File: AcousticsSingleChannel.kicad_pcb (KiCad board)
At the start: 4 copper layers, 25.4 x 25.4 mm, 35 parts, among them J1 Conn_01x04_Pin, J2 Conn_01x04_Pin, J4 Conn_01x09_Pin, U1 OPA1604AIPWR, U2 ADS127L21IRUKT, U3 LTC6910-3CTS8#TRPBF

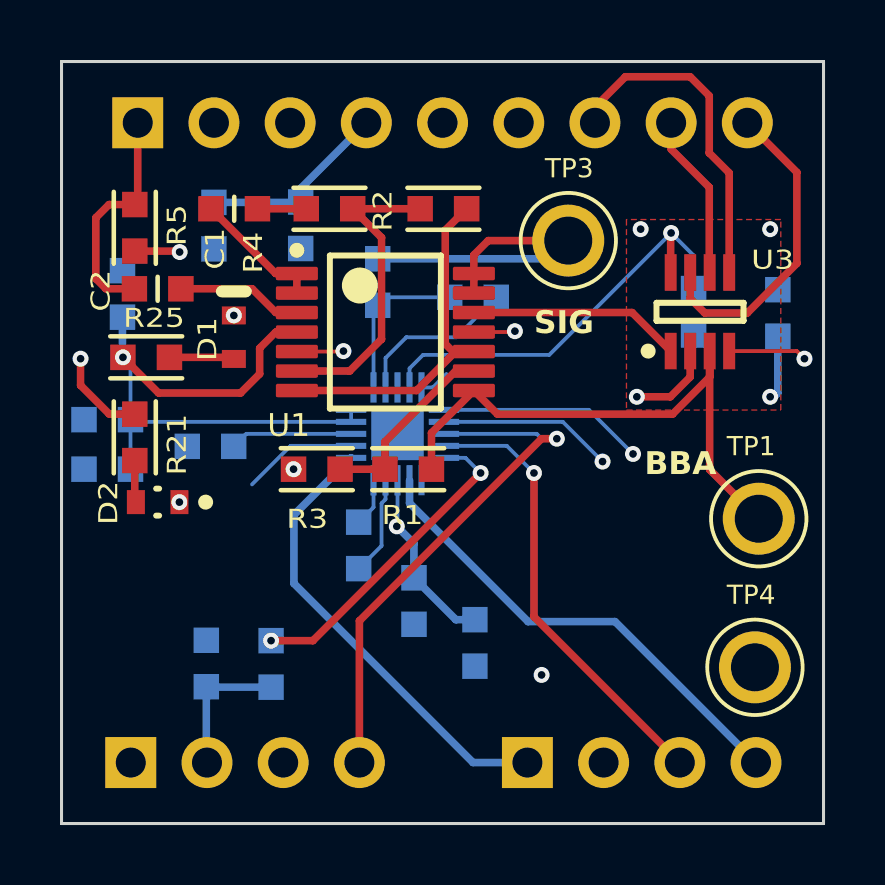
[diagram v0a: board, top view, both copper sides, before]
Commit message: tracks
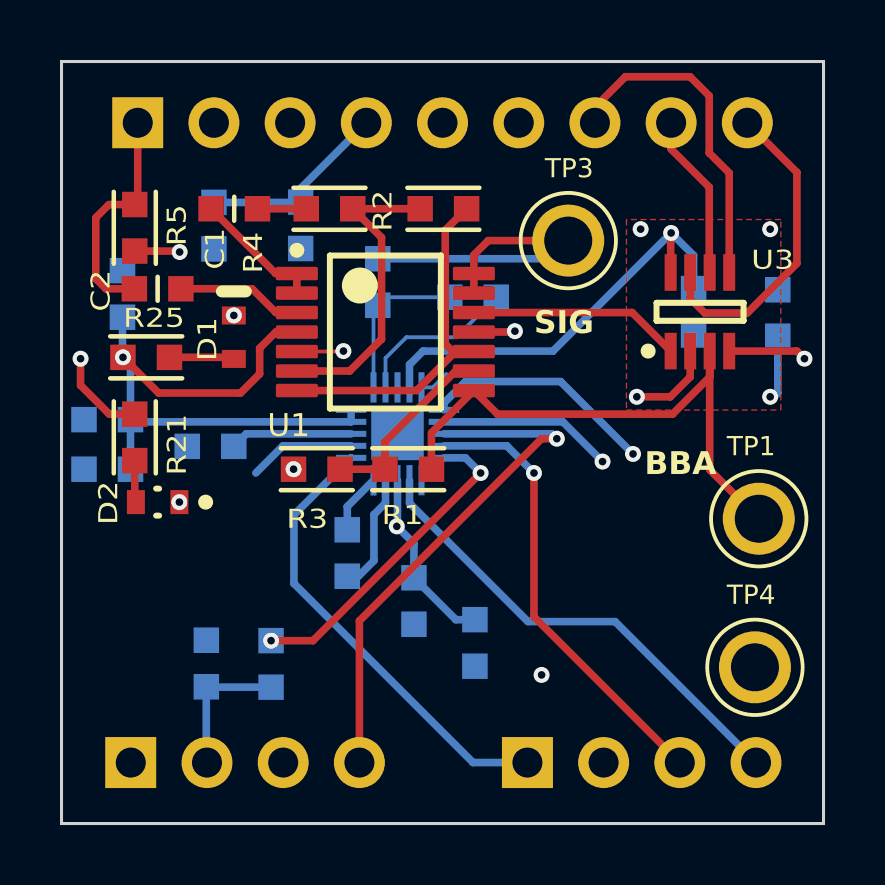
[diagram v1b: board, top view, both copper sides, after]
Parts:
- moved C4 0.46 mm to (138.3, 99.1)
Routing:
- net /RESET: track 23.8 -> 24.7 mm
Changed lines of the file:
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@@
 	(footprint "AltiumImports:SMD-0603C"
 		(layer "B.Cu")
-		(at 138.72206 98.855005 180)
+		(at 138.34106 99.109005 180)
 		(property "Reference" "C4"
 			(at 0.762 -0.635 0)
@@
 	)
 	(segment
-		(start 143.900359 91.743005)
-		(end 142.56106 91.743005)
-		(width 0.127)
+		(start 151.07106 92.378005)
+		(end 153.32706 92.378005)
+		(width 0.254)
 		(layer "F.Cu")
 		(net 1)
 	)
 	(segment
-		(start 143.92906 91.714304)
-		(end 143.900359 91.743005)
-		(width 0.127)
+		(start 143.900359 91.743005)
+		(end 143.92906 91.714304)
+		(width 0.254)
 		(layer "F.Cu")
 		(net 1)
 	)
 	(segment
-		(start 151.11798 92.424925)
-		(end 151.07106 92.378005)
+		(start 153.32706 92.378005)
+		(end 153.58106 92.632005)
 		(width 0.254)
 		(layer "F.Cu")
@@
 	)
 	(segment
-		(start 153.32706 92.378005)
+		(start 151.11798 92.424925)
 		(end 151.07106 92.378005)
-		(width 0.127)
+		(width 0.254)
 		(layer "F.Cu")
 		(net 1)
 	)
 	(segment
-		(start 153.58106 92.632005)
-		(end 153.32706 92.378005)
-		(width 0.127)
+		(start 142.56106 91.743005)
+		(end 143.900359 91.743005)
+		(width 0.254)
 		(layer "F.Cu")
 		(net 1)
@@
 	)
 	(segment
-		(start 138.72206 99.630005)
-		(end 139.48406 98.868005)
-		(width 0.127)
-		(layer "B.Cu")
-		(net 1)
-	)
-	(segment
 		(start 140.31056 91.916504)
 		(end 141.97456 91.916504)
@@
 	)
 	(segment
-		(start 139.48406 97.450006)
-		(end 139.615861 97.318205)
-		(width 0.127)
-		(layer "B.Cu")
-		(net 1)
-	)
-	(segment
 		(start 141.97456 91.916504)
 		(end 143.30706 90.584004)
@@
 	)
 	(segment
+		(start 138.70906 99.884005)
+		(end 139.23006 99.363005)
+		(width 0.254)
+		(layer "B.Cu")
+		(net 1)
+	)
+	(segment
 		(start 139.615861 93.589205)
 		(end 139.615861 92.611203)
@@
 	)
 	(segment
-		(start 136.452061 95.537004)
-		(end 135.16606 96.823005)
-		(width 0.127)
+		(start 139.23006 97.825807)
+		(end 139.615861 97.440006)
+		(width 0.254)
 		(layer "B.Cu")
 		(net 1)
 	)
 	(segment
-		(start 139.615861 97.318205)
+		(start 138.46806 95.537004)
+		(end 136.198061 95.537004)
+		(width 0.254)
+		(layer "B.Cu")
+		(net 1)
+	)
+	(segment
+		(start 139.615861 97.440006)
 		(end 139.615861 96.684805)
-		(width 0.127)
+		(width 0.254)
 		(layer "B.Cu")
 		(net 1)
 	)
 	(segment
-		(start 139.48406 98.868005)
-		(end 139.48406 97.450006)
-		(width 0.127)
+		(start 136.198061 95.537004)
+		(end 135.29306 96.442005)
+		(width 0.254)
 		(layer "B.Cu")
 		(net 1)
 	)
 	(segment
-		(start 138.46806 95.537004)
-		(end 136.452061 95.537004)
-		(width 0.127)
+		(start 138.34106 99.884005)
+		(end 138.70906 99.884005)
+		(width 0.254)
+		(layer "B.Cu")
+		(net 1)
+	)
+	(segment
+		(start 139.23006 99.363005)
+		(end 139.23006 97.825807)
+		(width 0.254)
 		(layer "B.Cu")
 		(net 1)
@@
 	)
 	(segment
-		(start 134.97306 95.137005)
-		(end 134.55706 95.553005)
-		(width 0.127)
+		(start 138.46806 95.137005)
+		(end 134.97306 95.137005)
+		(width 0.254)
 		(layer "B.Cu")
 		(net 6)
 	)
 	(segment
-		(start 138.46806 95.137005)
-		(end 134.97306 95.137005)
-		(width 0.127)
+		(start 134.97306 95.137005)
+		(end 134.55706 95.553005)
+		(width 0.254)
 		(layer "B.Cu")
 		(net 6)
 	)
 	(segment
-		(start 139.215859 96.684805)
-		(end 139.215859 97.586206)
-		(width 0.127)
+		(start 138.34106 97.559604)
+		(end 139.215859 96.684805)
+		(width 0.254)
 		(layer "B.Cu")
 		(net 7)
 	)
 	(segment
-		(start 139.215859 97.586206)
-		(end 138.72206 98.080005)
-		(width 0.127)
+		(start 138.34106 98.334005)
+		(end 138.34106 97.559604)
+		(width 0.254)
 		(layer "B.Cu")
 		(net 7)
@@
 		(start 143.659059 95.537004)
 		(end 144.56406 96.442005)
-		(width 0.127)
+		(width 0.254)
 		(layer "B.Cu")
 		(net 10)
@@
 		(start 141.56366 95.537004)
 		(end 143.659059 95.537004)
-		(width 0.127)
+		(width 0.254)
 		(layer "B.Cu")
 		(net 10)
@@
 		(start 141.56366 94.737006)
 		(end 145.526061 94.737006)
-		(width 0.127)
+		(width 0.254)
 		(layer "B.Cu")
 		(net 11)
@@
 		(start 145.526061 94.737006)
 		(end 146.85006 96.061005)
-		(width 0.127)
+		(width 0.254)
 		(layer "B.Cu")
 		(net 11)
@@
 	)
 	(segment
-		(start 144.81806 95.299005)
-		(end 144.65606 95.137005)
-		(width 0.127)
-		(layer "B.Cu")
-		(net 13)
-	)
-	(segment
-		(start 144.65606 95.137005)
-		(end 141.56366 95.137005)
-		(width 0.127)
+		(start 145.16406 95.137005)
+		(end 145.32606 95.299005)
+		(width 0.254)
 		(layer "B.Cu")
 		(net 13)
 	)
 	(segment
-		(start 145.32606 95.299005)
-		(end 144.81806 95.299005)
-		(width 0.127)
+		(start 141.56366 95.137005)
+		(end 145.16406 95.137005)
+		(width 0.254)
 		(layer "B.Cu")
 		(net 13)
@@
 	(segment
 		(start 141.56366 94.337004)
-		(end 146.396059 94.337004)
-		(width 0.127)
+		(end 141.56366 94.108405)
+		(width 0.254)
 		(layer "B.Cu")
 		(net 17)
 	)
 	(segment
-		(start 146.396059 94.337004)
+		(start 145.45306 93.394005)
 		(end 147.86606 95.807005)
-		(width 0.127)
+		(width 0.254)
+		(layer "B.Cu")
+		(net 17)
+	)
+	(segment
+		(start 142.27806 93.394005)
+		(end 145.45306 93.394005)
+		(width 0.254)
+		(layer "B.Cu")
+		(net 17)
+	)
+	(segment
+		(start 141.56366 94.108405)
+		(end 142.27806 93.394005)
+		(width 0.254)
 		(layer "B.Cu")
 		(net 17)
@@
 	)
 	(segment
-		(start 140.01586 96.684805)
-		(end 140.01586 98.196205)
-		(width 0.127)
+		(start 140.01586 98.196205)
+		(end 139.99206 98.220005)
+		(width 0.254)
 		(layer "B.Cu")
 		(net 20)
@@
 	)
 	(segment
-		(start 140.01586 98.196205)
-		(end 139.99206 98.220005)
-		(width 0.127)
+		(start 140.01586 96.684805)
+		(end 140.01586 98.196205)
+		(width 0.254)
 		(layer "B.Cu")
 		(net 20)
@@
 	)
 	(segment
-		(start 142.281061 95.937006)
-		(end 141.56366 95.937006)
-		(width 0.127)
+		(start 141.56366 95.937006)
+		(end 142.281061 95.937006)
+		(width 0.254)
 		(layer "B.Cu")
 		(net 26)
 	)
 	(segment
-		(start 142.78606 96.442005)
-		(end 142.281061 95.937006)
-		(width 0.127)
+		(start 142.281061 95.937006)
+		(end 142.78606 96.442005)
+		(width 0.254)
 		(layer "B.Cu")
 		(net 26)
@@
 	)
 	(segment
-		(start 138.46806 94.737006)
-		(end 131.188061 94.737006)
-		(width 0.127)
+		(start 133.89606 87.422165)
+		(end 136.776088 87.422165)
+		(width 0.254)
 		(layer "B.Cu")
 		(net 29)
@@
 		(start 131.188061 94.737006)
 		(end 131.11506 94.664005)
-		(width 0.127)
+		(width 0.254)
 		(layer "B.Cu")
 		(net 29)
 	)
 	(segment
-		(start 133.89606 87.422165)
-		(end 136.776088 87.422165)
+		(start 138.46806 94.737006)
+		(end 131.188061 94.737006)
 		(width 0.254)
 		(layer "B.Cu")
@@
 	)
 	(segment
-		(start 145.07206 92.505005)
-		(end 149.13606 88.441005)
-		(width 0.127)
+		(start 131.11506 96.315005)
+		(end 131.11506 94.664005)
+		(width 0.254)
 		(layer "B.Cu")
 		(net 29)
 	)
 	(segment
-		(start 149.88506 89.190005)
-		(end 149.13606 88.441005)
-		(width 0.127)
+		(start 130.84806 92.571005)
+		(end 130.86406 92.587005)
+		(width 0.254)
 		(layer "B.Cu")
 		(net 29)
 	)
 	(segment
-		(start 130.84806 92.571005)
-		(end 130.86406 92.587005)
+		(start 149.88506 90.293005)
+		(end 149.88506 89.190005)
 		(width 0.254)
 		(layer "B.Cu")
@@
 	)
 	(segment
-		(start 140.866659 92.505005)
-		(end 145.07206 92.505005)
-		(width 0.127)
+		(start 131.11506 92.838005)
+		(end 130.86406 92.587005)
+		(width 0.254)
 		(layer "B.Cu")
 		(net 29)
@@
 	)
 	(segment
-		(start 131.11506 92.838005)
-		(end 130.86406 92.587005)
-		(width 0.127)
+		(start 149.88506 89.190005)
+		(end 149.13606 88.441005)
+		(width 0.254)
 		(layer "B.Cu")
 		(net 29)
 	)
 	(segment
-		(start 140.415859 93.589205)
-		(end 140.415859 92.955805)
-		(width 0.127)
+		(start 140.866659 92.378005)
+		(end 145.19906 92.378005)
+		(width 0.254)
 		(layer "B.Cu")
 		(net 29)
@@
 	(segment
 		(start 131.11506 94.664005)
-		(end 131.11506 96.315005)
-		(width 0.127)
+		(end 131.11506 92.838005)
+		(width 0.254)
 		(layer "B.Cu")
 		(net 29)
 	)
 	(segment
-		(start 140.415859 92.955805)
-		(end 140.866659 92.505005)
-		(width 0.127)
+		(start 140.415859 93.589205)
+		(end 140.415859 92.828805)
+		(width 0.254)
 		(layer "B.Cu")
 		(net 29)
 	)
 	(segment
-		(start 138.46806 94.337004)
-		(end 138.46806 94.737006)
-		(width 0.127)
+		(start 140.415859 92.828805)
+		(end 140.866659 92.378005)
+		(width 0.254)
 		(layer "B.Cu")
 		(net 29)
 	)
 	(segment
-		(start 131.11506 94.664005)
-		(end 131.11506 92.838005)
-		(width 0.127)
+		(start 145.19906 92.378005)
+		(end 149.13606 88.441005)
+		(width 0.254)
 		(layer "B.Cu")
 		(net 29)
 	)
 	(segment
-		(start 149.88506 90.293005)
-		(end 149.88506 89.190005)
-		(width 0.127)
+		(start 138.46806 94.337004)
+		(end 138.46806 94.737006)
+		(width 0.254)
 		(layer "B.Cu")
 		(net 29)
